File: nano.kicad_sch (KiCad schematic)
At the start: 5 parts

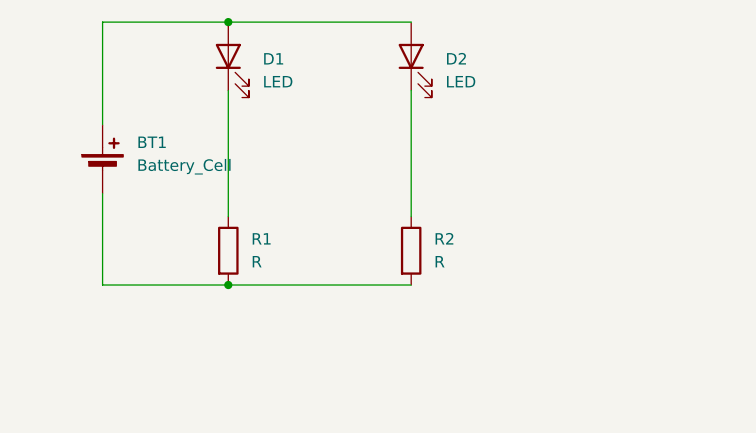
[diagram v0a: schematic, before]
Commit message: Final
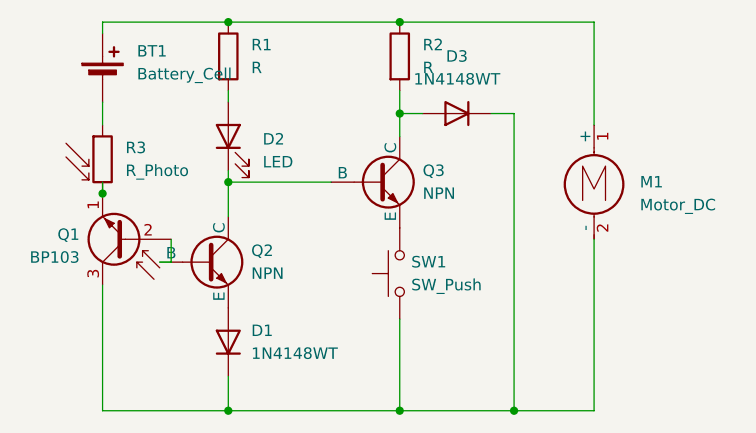
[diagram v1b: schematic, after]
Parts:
- removed D1: LED, LED_THT:LED_D5.0mm, symbol Device:LED
- added D1, D3: 1N4148WT, Diode_SMD:D_SOD-523, symbol Diode:1N4148WT
- added M1: Motor_DC, Motors:Vybronics_VZ30C1T8219732L, symbol Motor:Motor_DC
- added Q1: BP103, Package_TO_SOT_THT:TO-18-3_Lens, symbol Sensor_Optical:BP103
- added Q2, Q3: NPN, Package_TO_SOT_THT:TO-92L_HandSolder, symbol Simulation_SPICE:NPN
- added R3: R_Photo, OptoDevice:R_LDR_5.1x4.3mm_P3.4mm_Vertical, symbol Device:R_Photo
- added SW1: SW_Push, Button_Switch_THT:SW_PUSH_6mm, symbol Switch:SW_Push
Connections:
- net at BT1.1 (+): now also R1.1, R2.1, M1.1 (+); no longer D2.2 (A)
- net at D2.1 (K): now also Q2.1 (C), Q3.2 (B); no longer R2.1
- new net: BT1.2 (-), R3.1
- new net: Q1.1 (E), R3.2
- new net: Q1.2 (B), Q2.2 (B)
- new net: D1.1 (K), D3.1 (K), M1.2 (-), Q1.3 (C), SW1.1
- new net: D3.2 (A), Q3.1 (C), R2.2
- new net: Q3.3 (E), SW1.2
- new net: D2.2 (A), R1.2
- new net: D1.2 (A), Q2.3 (E)
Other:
- moved on the sheet: BT1, D2, R1, R2
